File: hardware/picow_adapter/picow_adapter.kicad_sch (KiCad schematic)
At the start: 1 part

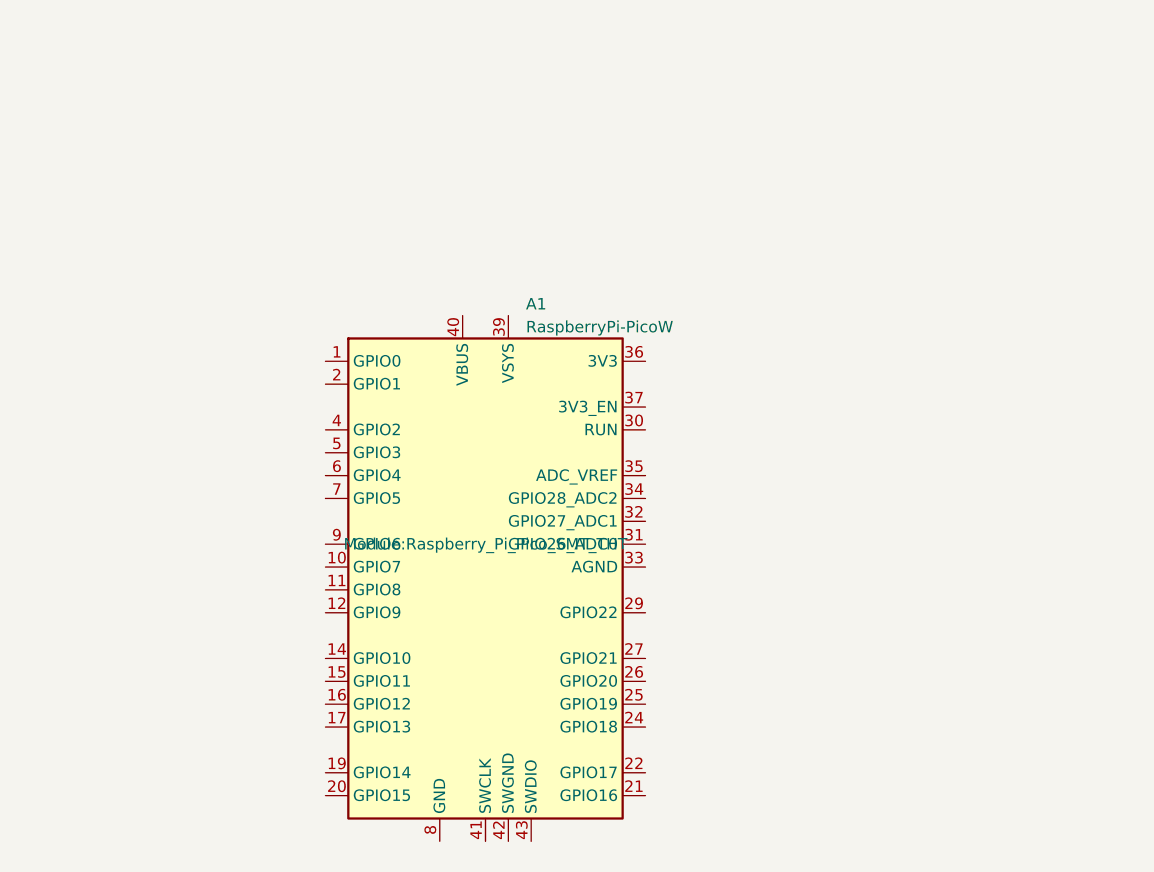
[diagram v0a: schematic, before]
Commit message: update
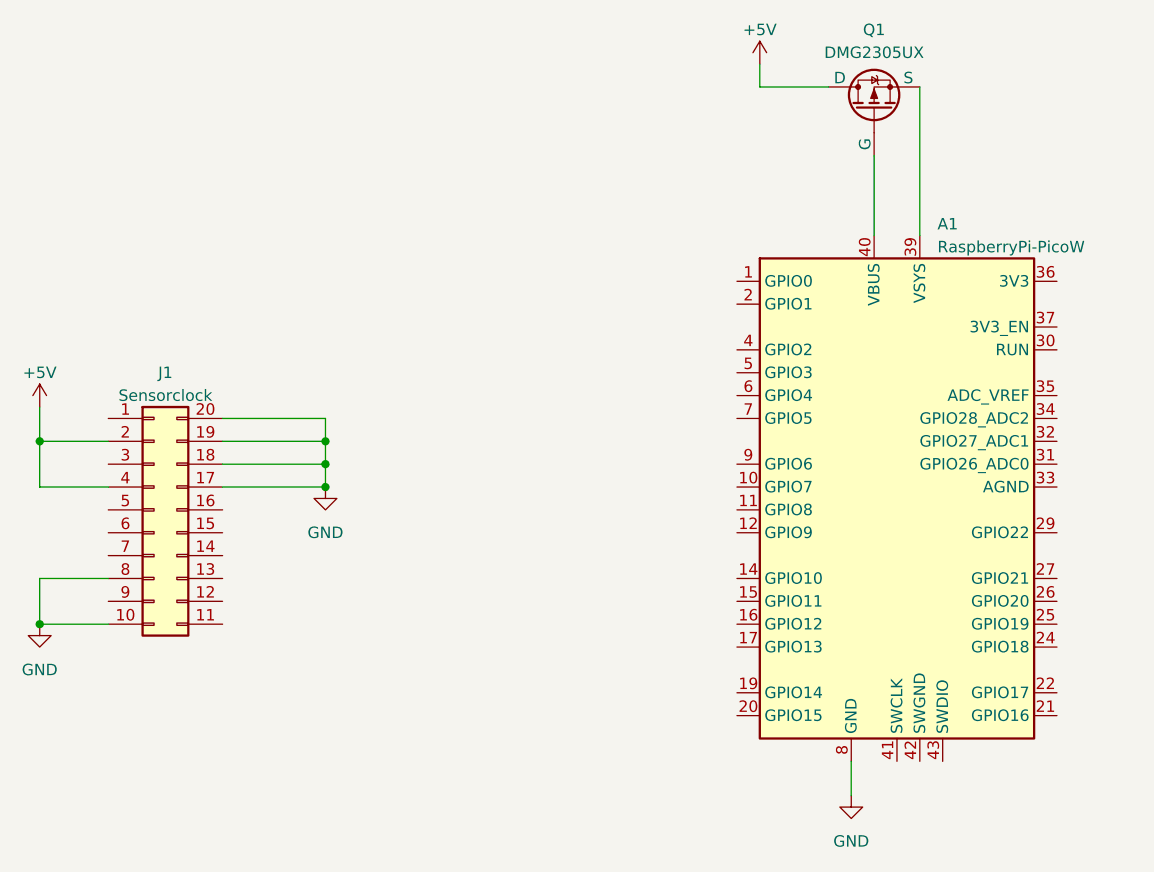
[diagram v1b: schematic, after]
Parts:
- added J1: Sensorclock, symbol Connector_Generic:Conn_02x10_Counter_Clockwise
- added Q1: DMG2305UX, Package_TO_SOT_SMD:SOT-23, symbol Simulation_SPICE:PMOS
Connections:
- net GND: now reaches A1.13 (GND), A1.18 (GND), A1.23 (GND), A1.28 (GND), A1.3 (GND), A1.38 (GND), A1.8 (GND)
- net GND: now also J1.10 (Pin_10), J1.17 (Pin_17), J1.18 (Pin_18), J1.19 (Pin_19), J1.20 (Pin_20), J1.8 (Pin_8)
- net at A1.39 (VSYS): now also Q1.2 (S)
- net at A1.40 (VBUS): now also Q1.1 (G)
- new net +5V: J1.2 (Pin_2), J1.4 (Pin_4), Q1.3 (D)
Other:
- moved on the sheet: A1
